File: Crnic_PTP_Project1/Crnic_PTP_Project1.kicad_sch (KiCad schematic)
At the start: 24 parts, among them U1 NE555P, U2 LM2574N-5

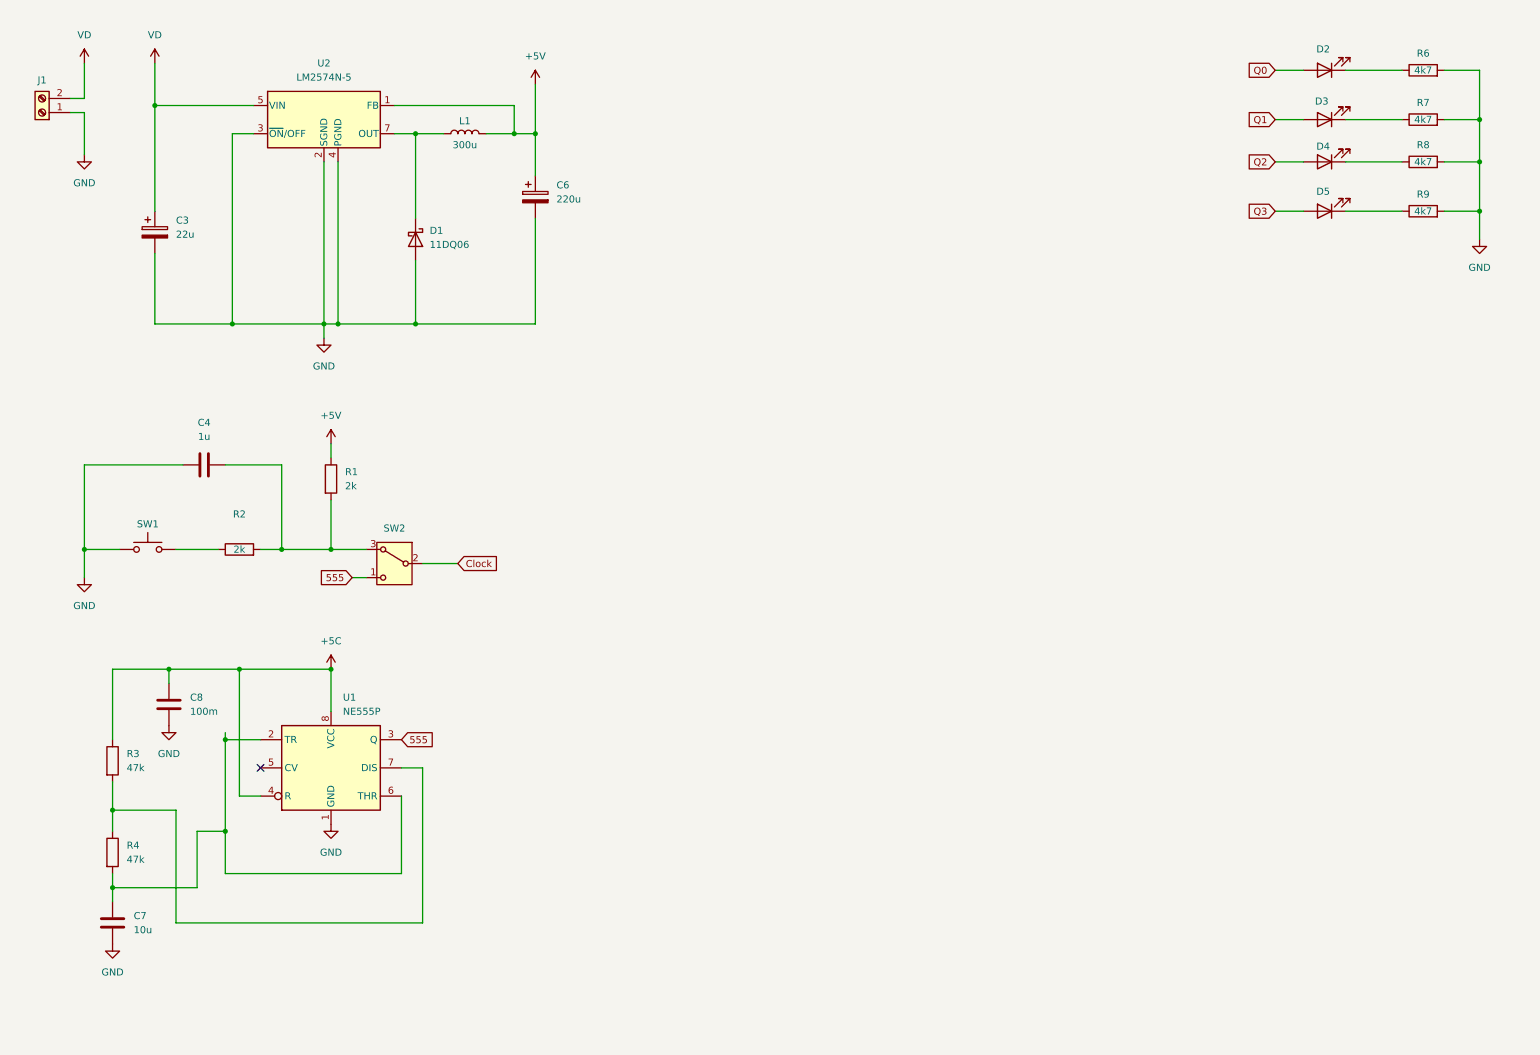
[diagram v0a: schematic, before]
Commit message: routanje
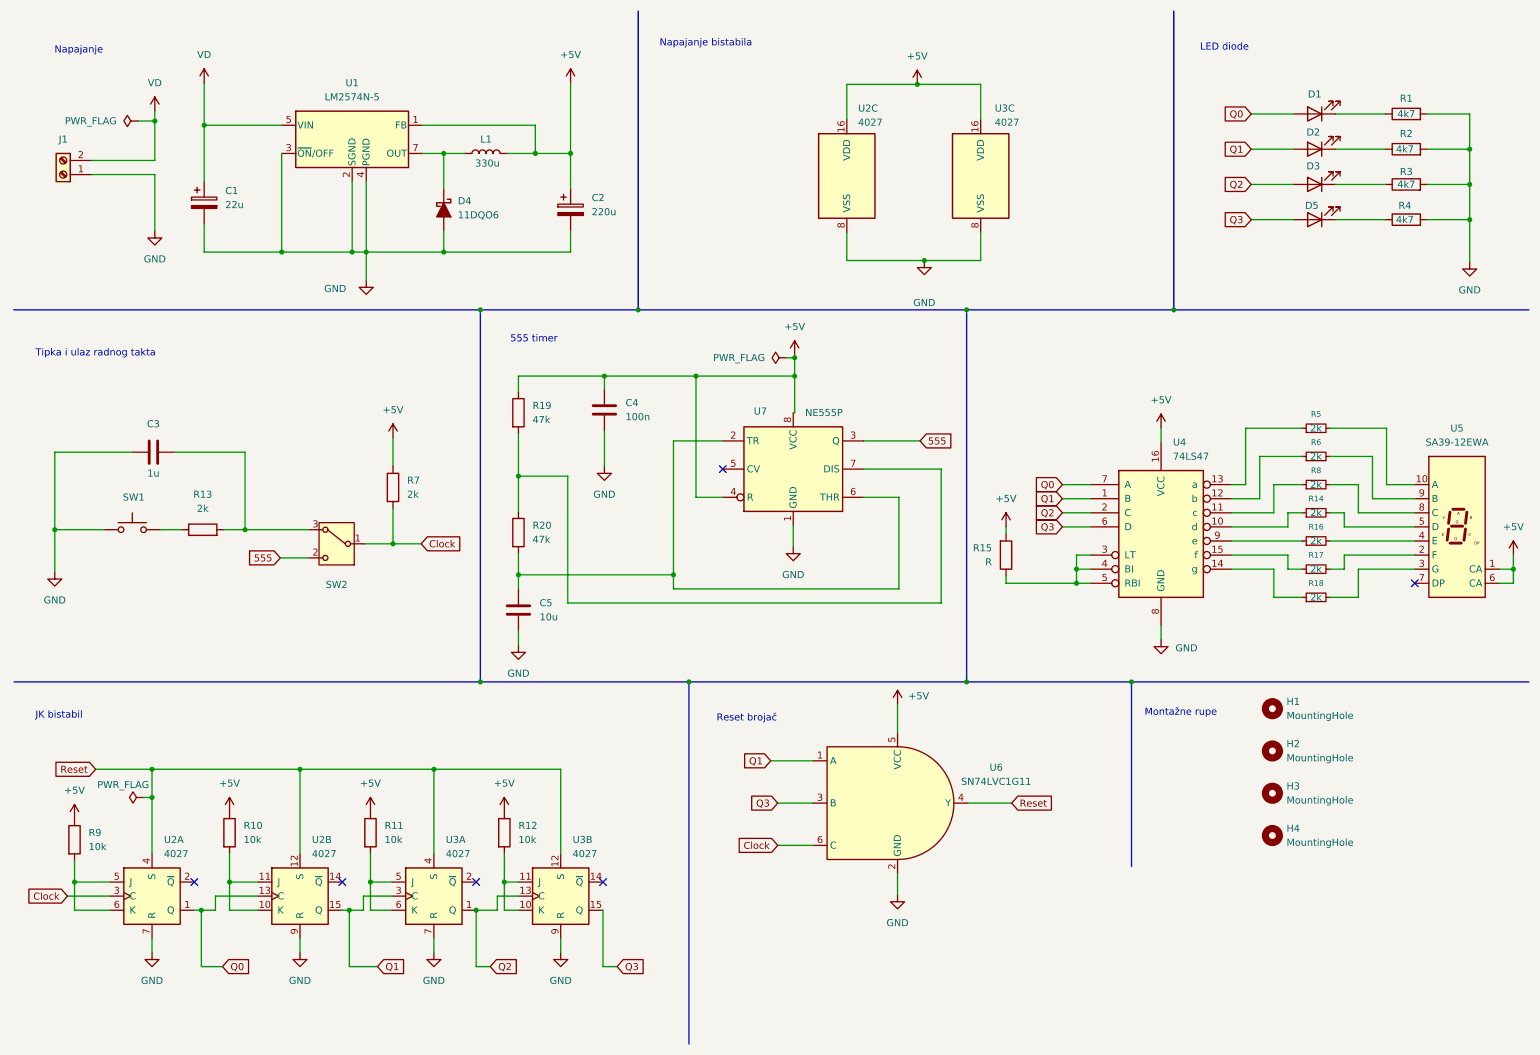
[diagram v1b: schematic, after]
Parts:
- removed C3: 22u, symbol Device:C_Polarized
- removed C6: 220u, symbol Device:C_Polarized
- removed C7: 10u, symbol Device:C
- removed C8: 100m, symbol Device:C
- removed D1: 11DQ06, symbol Device:D_Schottky
- removed D4: ~, symbol Device:LED
- removed R6, R8: 4k7, symbol Device:R
- removed SW1: ~, symbol Switch:SW_MEC_5G
- removed SW2: ~, Button_Switch_SMD:Nidec_Copal_CAS-120A, symbol Switch:SW_Nidec_CAS-120A1
- removed U1: NE555P, Package_DIP:DIP-8_W7.62mm, symbol Timer:NE555P
- removed U2: LM2574N-5, Package_DIP:DIP-8_W7.62mm, symbol Regulator_Switching:LM2574N-5
- added C1: 22u, Capacitor_THT:CP_Radial_D5.0mm_P2.00mm, symbol Device:C_Polarized
- added C2: 220u, Capacitor_THT:CP_Radial_D5.0mm_P2.00mm, symbol Device:C_Polarized
- added C3: 1u, Capacitor_SMD:C_1206_3216Metric_Pad1.33x1.80mm_HandSolder, symbol Device:C
- added C5: 10u, Capacitor_SMD:C_1206_3216Metric_Pad1.33x1.80mm_HandSolder, symbol Device:C
- added D1: ~, LED_THT:LED_D5.0mm, symbol Device:LED
- added D4: 11DQO6, Diode_THT:D_DO-41_SOD81_P12.70mm_Horizontal, symbol Device:D_Schottky_Filled
- added H1, H2, H3, H4: MountingHole, MountingHole:MountingHole_5.5mm, symbol Mechanical:MountingHole
- added R10, R11, R12: 10k, Resistor_SMD:R_1206_3216Metric_Pad1.30x1.75mm_HandSolder, symbol Device:R
- added R13: 2k, Resistor_SMD:R_1206_3216Metric_Pad1.30x1.75mm_HandSolder, symbol Device:R
- added R14, R16, R17, R18, R5, R6, R8: 2k, Resistor_SMD:R_1206_3216Metric_Pad1.30x1.75mm_HandSolder, symbol Device:R_Small
- added R15: R, Resistor_SMD:R_1206_3216Metric_Pad1.30x1.75mm_HandSolder, symbol Device:R
- added R19, R20: 47k, Resistor_SMD:R_1206_3216Metric_Pad1.30x1.75mm_HandSolder, symbol Device:R
- added SW1: ~, Button_Switch_THT:SW_PUSH_6mm_H4.3mm, symbol Switch:SW_Push
- added SW2: ~, Button_Switch_THT:SW_Slide_SPDT_Straight_CK_OS102011MS2Q, symbol Switch:SW_SPDT_312
- added U1: LM2574N-5, Package_DIP:DIP-8_W7.62mm_Socket_LongPads, symbol Regulator_Switching:LM2574N-5
- added U2, U3: 4027, Package_DIP:DIP-16_W7.62mm_Socket_LongPads, symbol 4xxx:4027
- added U4: 74LS47, Package_DIP:DIP-16_W7.62mm_Socket_LongPads, symbol 74xx:74LS47
- added U5: SA39-12EWA, Display_7Segment:HDSP-7401, symbol Display_Character:SA39-12EWA
- added U6: SN74LVC1G11, Package_TO_SOT_SMD:SOT-23-6, symbol SN74LVC1G11:SN74LVC1G11
- added U7: NE555P, Package_DIP:DIP-8_W7.62mm, symbol Timer:NE555P
- C4: value 1u -> 100n; footprint (none) -> Capacitor_SMD:C_1206_3216Metric_Pad1.33x1.80mm_HandSolder
- D2, D3, D5: footprint (none) -> LED_THT:LED_D5.0mm
- J1: footprint (none) -> TerminalBlock_MetzConnect:TerminalBlock_MetzConnect_Type011_RT05502HBLC_1x02_P5.00mm_Horizontal
- L1: value 300u -> 330u; footprint (none) -> Inductor_THT:L_Radial_D7.2mm_P3.00mm_Murata_1700
- R1, R2: value 2k -> 4k7; footprint (none) -> Resistor_THT:R_Axial_DIN0207_L6.3mm_D2.5mm_P10.16mm_Horizontal
- R3, R4: value 47k -> 4k7; footprint (none) -> Resistor_THT:R_Axial_DIN0207_L6.3mm_D2.5mm_P10.16mm_Horizontal
- R7: value 4k7 -> 2k; footprint (none) -> Resistor_SMD:R_1206_3216Metric_Pad1.30x1.75mm_HandSolder
- R9: value 4k7 -> 10k; footprint (none) -> Resistor_SMD:R_1206_3216Metric_Pad1.30x1.75mm_HandSolder
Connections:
- net +5C is gone; now on an unnamed net: R3.1
- net +5V: now also C4.1, R7.1, R9.1, C2.1, R10.1, R11.1, R12.1, R15.2, R19.1, U1.1 (FB), U2.16 (VDD), U3.16 (VDD), U4.16 (VCC), U5.1 (CA), U5.6 (CA), U6.5 (VCC), U7.4 (R), U7.8 (VCC); no longer R1.1
- net 555: now also SW2.2 (A), U7.3 (Q)
- net Clock: now also R7.2, SW2.1 (B), U2.3 (C), U6.6 (C)
- net GND: now also C4.2, R1.2, R2.2, R3.2, R4.2, C1.2, C2.2, C3.1, C5.2, D4.2 (A), SW1.1, U1.2 (SGND), U1.3 (~{ON}/OFF), U1.4 (PGND), U2.7 (R), U2.8 (VSS), U2.9 (R), U3.7 (R), U3.8 (VSS), U3.9 (R), U4.8 (GND), U6.2 (GND), U7.1 (GND); no longer C4.1, R7.2, R9.2
- net Q0: now also D1.2 (A), U2.1 (Q), U2.13 (C), U4.7 (A); no longer D2.2 (A)
- net Q1: now also D2.2 (A), U2.15 (Q), U3.3 (C), U4.1 (B), U6.1 (A); no longer D3.2 (A)
- net Q2: now also D3.2 (A), U3.1 (Q), U3.13 (C), U4.2 (C)
- net Q3: now also U3.15 (Q), U4.6 (D), U6.3 (B)
- net VD: now also C1.1, U1.5 (VIN)
- net at D3.1 (K): no longer R7.1
- net at L1.1: now also D4.1 (K), U1.7 (OUT)
- net at D2.1 (K): now also R2.1
- net at D5.1 (K): now also R4.1; no longer R9.1
- new net: R5.1, U4.13 (a)
- new net: R5.2, U5.10 (A)
- new net: R11.2, U3.5 (J), U3.6 (K)
- new net: R17.1, U4.15 (f)
- new net: R17.2, U5.2 (F)
- new net: R19.2, R20.1, U7.7 (DIS)
- new net: C5.1, R20.2, U7.2 (TR), U7.6 (THR)
- new net: R9.2, U2.5 (J), U2.6 (K)
- new net: R18.2, U5.3 (G)
- new net: R16.2, U5.4 (E)
- new net: R14.2, U5.5 (D)
- new net: R8.2, U5.8 (C)
- new net: R6.2, U5.9 (B)
- new net: R6.1, U4.12 (b)
- new net: C3.2, R13.2, SW2.3 (C)
- new net: R13.1, SW1.2
- new net: D1.1 (K), R1.1
- new net: R14.1, U4.10 (d)
- new net: R8.1, U4.11 (c)
- new net: R18.1, U4.14 (g)
- new net: R15.1, U4.3 (LT), U4.4 (BI), U4.5 (RBI)
- new net: R16.1, U4.9 (e)
- new net: R10.2, U2.10 (K), U2.11 (J)
- new net: R12.2, U3.10 (K), U3.11 (J)
- new net Reset: U2.12 (S), U2.4 (S), U3.12 (S), U3.4 (S), U6.4 (Y)
- no-connect marks 1 -> 6
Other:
- note added: "555 timer"
- note added: "JK bistabil"
- note added: "LED diode"
- note added: "Montažne rupe"
- note added: "Napajanje"
- note added: "Napajanje bistabila"
- note added: "Reset brojač"
- note added: "Tipka i ulaz radnog takta"
